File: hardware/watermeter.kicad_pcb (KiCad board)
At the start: 2 copper layers, 100.3 x 49.5 mm, 46 parts, among them J1 flow_meter, J2 t_in, J3 t_out, J4 USB-TYPE-C-31-M-12, J9 24V_Power, SW1 Reboot, U1 K7805-500R3, U2 ESP32-C6-MINI-1, U3 USBLC6-2SC6, U4 LM3671MFX-3.3/NOPB

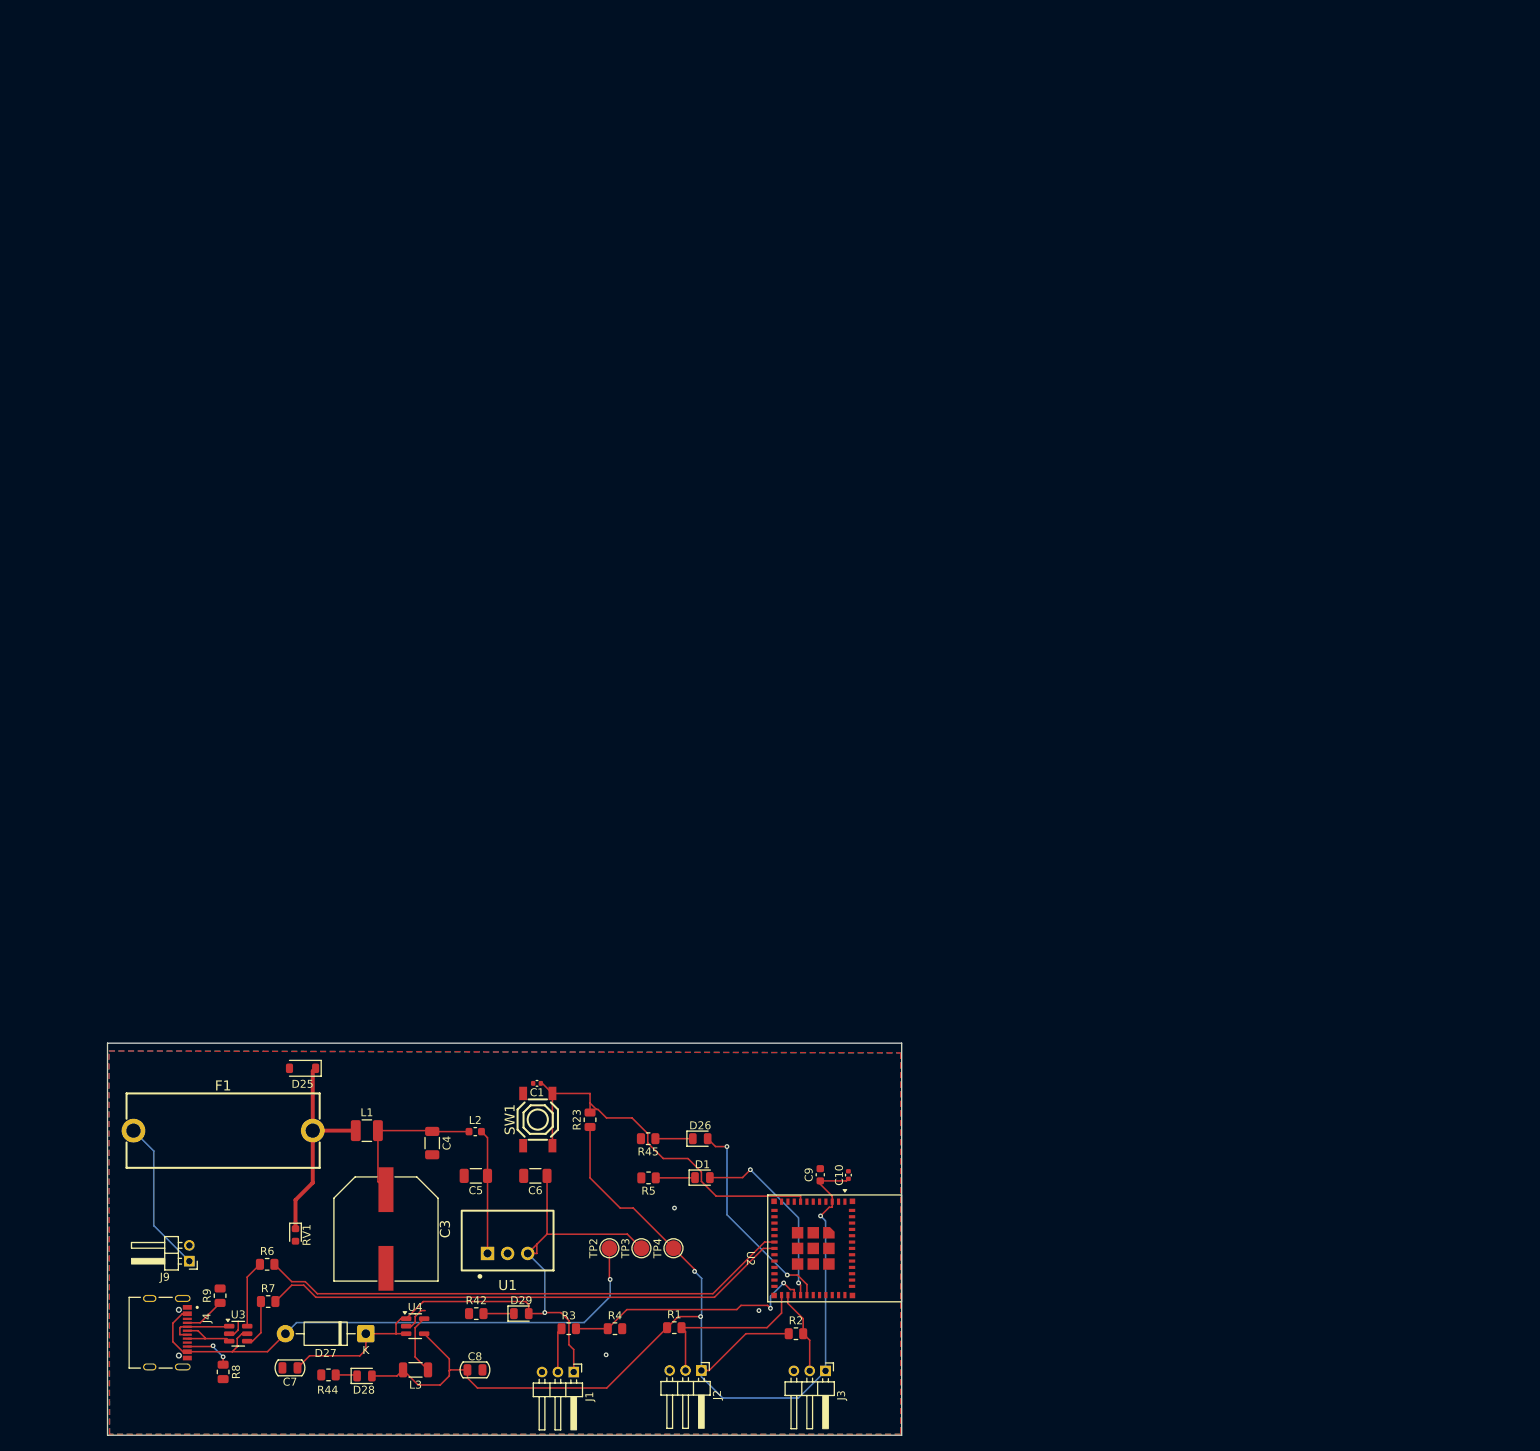
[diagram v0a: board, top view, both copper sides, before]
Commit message: Refactoring
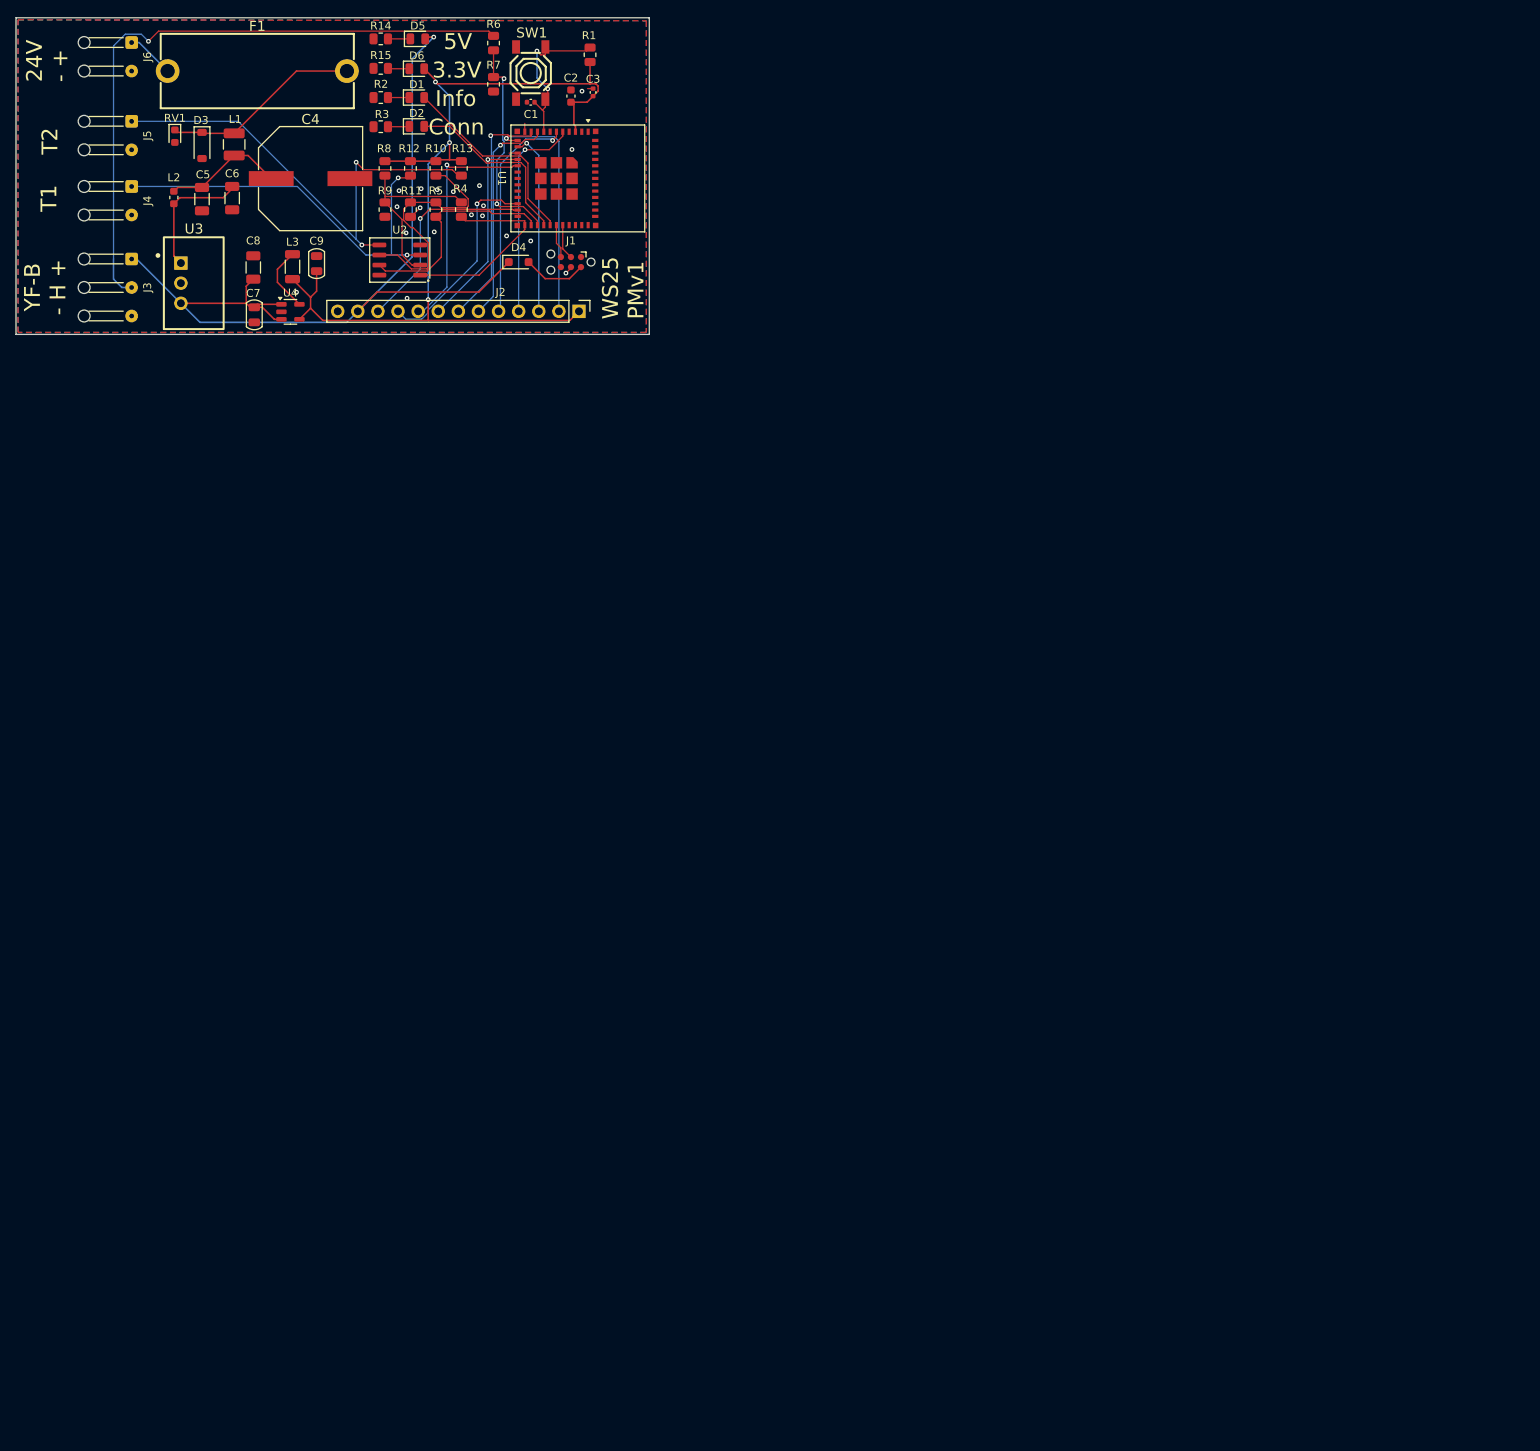
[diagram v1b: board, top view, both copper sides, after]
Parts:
- removed C10: 0.1uF, Capacitor_SMD:C_0402_1005Metric
- removed D25: BAT46W, Diode_SMD:D_SOD-123
- removed D26, D28, D29: KT-0805G, LED_SMD:LED_0805_2012Metric
- removed D27: 1N5819, Diode_THT:D_DO-41_SOD81_P10.16mm_Horizontal
- removed J9: 24V_Power, Connector_PinHeader_2.00mm:PinHeader_1x02_P2.00mm_Horizontal
- removed R23: 10K, Resistor_SMD:R_0805_2012Metric
- removed R42, R44, R45: 20R, Resistor_SMD:R_0805_2012Metric
- removed TP2: 5V_USB, TestPoint:TestPoint_Pad_D2.0mm
- removed TP3: 5V, TestPoint:TestPoint_Pad_D2.0mm
- removed TP4: 3.3V, TestPoint:TestPoint_Pad_D2.0mm
- added C2: 22uF, Capacitor_SMD:C_0603_1608Metric, F.Cu at (70.1, 9.89)
- added D2: KT-0805B, Diode_SMD:D_0805_2012Metric, F.Cu at (50.6, 13.7)
- added D3: BAT46W, Diode_SMD:D_SOD-123, F.Cu at (23.5, 16.1)
- added D4: 1N5819, Diode_SMD:D_SOD-323_HandSoldering, F.Cu at (63.5, 30.9)
- added D5: KT-0805G, LED_SMD:LED_0805_2012Metric, F.Cu at (50.8, 2.67)
- added D6: KT-0805G, LED_SMD:LED_0805_2012Metric, F.Cu at (50.6, 6.44)
- added J5: PT1000-2, Connector_Wire:SolderWire-0.1sqmm_1x02_P3.6mm_D0.4mm_OD1mm_Relief, F.Cu at (14.6, 13.1)
- added J6: 24V_Power, Connector_Wire:SolderWire-0.1sqmm_1x02_P3.6mm_D0.4mm_OD1mm_Relief, F.Cu at (14.6, 3.13)
- added R10: 4k7, Resistor_SMD:R_0805_2012Metric, F.Cu at (53.0, 19.0)
- added R11: 1k, Resistor_SMD:R_0805_2012Metric, F.Cu at (49.8, 24.2)
- added R12: 4k7, Resistor_SMD:R_0805_2012Metric, F.Cu at (49.8, 19.0)
- added R13: 4k7, Resistor_SMD:R_0805_2012Metric, F.Cu at (56.3, 19.0)
- added R14: 20R, Resistor_SMD:R_0805_2012Metric, F.Cu at (46.1, 2.67)
- added R15: 20R, Resistor_SMD:R_0805_2012Metric, F.Cu at (46.1, 6.39)
- C3: value 680uF/50V -> 0.1uF; footprint MyFootprints:CAP-SMD_BD12.5-L13.0-W13.0-LS14.4-FD -> Capacitor_SMD:C_0402_1005Metric
- C4: value 4.7uF/63V -> 680uF/50V; footprint Capacitor_SMD:C_1206_3216Metric -> MyFootprints:CAP-SMD_BD12.5-L13.0-W13.0-LS14.4-FD
- C5: value 10uF/50V -> 4.7uF/63V
- C6: value 22uF/10V -> 10uF/50V
- C8: value 10uF -> 22uF/10V; footprint PCM_Capacitor_SMD_AKL:C_0805_2012Metric -> Capacitor_SMD:C_1206_3216Metric
- C9: value 22uF -> 10uF; footprint Capacitor_SMD:C_0603_1608Metric -> PCM_Capacitor_SMD_AKL:C_0805_2012Metric
- D1: value KT-0805B -> KT-0805G; footprint Diode_SMD:D_0805_2012Metric -> LED_SMD:LED_0805_2012Metric
- J1: value flow_meter -> TC2030; footprint Connector_PinHeader_2.00mm:PinHeader_1x03_P2.00mm_Horizontal -> Connector:Tag-Connect_TC2030-IDC-NL_2x03_P1.27mm_Vertical
- J2: value t_in -> EXT; footprint Connector_PinHeader_2.00mm:PinHeader_1x03_P2.00mm_Horizontal -> Connector_PinHeader_2.54mm:PinHeader_1x13_P2.54mm_Vertical
- J3: value t_out -> flow_meter; footprint Connector_PinHeader_2.00mm:PinHeader_1x03_P2.00mm_Horizontal -> Connector_Wire:SolderWire-0.1sqmm_1x03_P3.6mm_D0.4mm_OD1mm_Relief
- J4: value USB-TYPE-C-31-M-12 -> PT1000-1; footprint MyFootprints:USB-HRO_TYPE-C-31-M-12 -> Connector_Wire:SolderWire-0.1sqmm_1x02_P3.6mm_D0.4mm_OD1mm_Relief
- R1: value 3.3k -> 10K
- R2: value 3.3k -> 20R
- R3: value 1k -> 15R
- R4: value 2k -> 20k
- R5: value 15R -> 20k
- R6: value 22R -> 1k
- R7: value 22R -> 2k
- R8: value 5.1 -> 4k7
- R9: value 5.1 -> 1k
- U1: value K7805-500R3 -> ESP32-C6-MINI-1; footprint MyFootprints:PWRM-TH_K78XX-500R3 -> RF_Module:ESP32-C6-MINI-1
- U2: value ESP32-C6-MINI-1 -> TLV2462AID; footprint RF_Module:ESP32-C6-MINI-1 -> PCM_Package_SO_AKL:SO-8_3.9x4.9mm_P1.27mm
- U3: value USBLC6-2SC6 -> K7805-500R3; footprint Package_TO_SOT_SMD:SOT-23-6 -> MyFootprints:PWRM-TH_K78XX-500R3
- moved J3 165.6 mm to (14.6, 30.5)
- moved R2 164.7 mm to (46.1, 10.1), turned to 180 degrees
- moved R1 161.2 mm to (72.5, 4.68), turned to 90 degrees
- moved R6 156.9 mm to (60.3, 3.20), turned to -90 degrees
- moved R7 156.4 mm to (60.3, 8.41), turned to -90 degrees
- moved R3 153.7 mm to (46.1, 13.8), turned to 180 degrees
- moved R8 153.4 mm to (46.6, 19.0)
- moved C3 146.0 mm to (72.9, 9.43), turned to 90 degrees
- moved J4 144.8 mm to (14.6, 21.3)
- moved R4 142.7 mm to (56.3, 24.2), turned to -90 degrees
- moved C8 142.1 mm to (30.0, 31.5), turned to 90 degrees
- moved D1 141.1 mm to (50.6, 10.1)
- moved L3 140.2 mm to (34.9, 31.4), turned to -90 degrees
- moved J1 140.2 mm to (70.1, 30.9), turned to 180 degrees
- moved RV1 139.6 mm to (20.1, 15.0)
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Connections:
- C1 pad 1: Net-(U2-EN) -> Net-(U1-EN)
- C3 pad 1: Net-(C3-Pad1) -> +3.3V
- C4 pad 1: Net-(C3-Pad1) -> Net-(C4-Pad1)
- C5 pad 1: Net-(U1-IN) -> Net-(C4-Pad1)
- C6 pad 1: +5V -> Net-(U3-IN)
- C8 pad 1: +3.3V -> +5V
- F1 pad 1: Net-(J9-Pin_1) -> /Power/24V
- J1 pad 1: +5V -> /EN
- J1 pad 2: Net-(J1-Pin_2) -> /5V_USB
- J1 pad 3: GND -> /TXD
- J2 pad 3: GND -> Net-(J2-Pin_3)
- J3 pad 1: +3.3V -> +5V
- L1 pad 2: Net-(C3-Pad1) -> Net-(C4-Pad1)
- L2 pad 1: Net-(C3-Pad1) -> Net-(C4-Pad1)
- L2 pad 2: Net-(U1-IN) -> Net-(U3-IN)
- R1 pad 2: Net-(J2-Pin_2) -> Net-(U1-EN)
- R2 pad 1: +3.3V -> Net-(D1-K)
- R2 pad 2: Net-(J3-Pin_2) -> GND
- R3 pad 1: Net-(J1-Pin_2) -> Net-(D2-K)
- R3 pad 2: Net-(U2-IO21) -> GND
- R4 pad 1: Net-(U2-IO21) -> Net-(U2A--)
- R4 pad 2: GND -> Net-(U1-IO19)
- R5 pad 1: Net-(D1-K) -> Net-(U2B--)
- R5 pad 2: GND -> Net-(U1-IO20)
- R6 pad 1: Net-(R6-Pad1) -> Net-(J3-Pin_2)
- R6 pad 2: /USB_D_N -> Net-(U1-IO21)
- R7 pad 1: Net-(R7-Pad1) -> Net-(U1-IO21)
- R7 pad 2: /USB_D_P -> GND
- R8 pad 1: Net-(J4-CC2) -> +3.3V
- R8 pad 2: GND -> Net-(U2A--)
- R9 pad 1: Net-(J4-CC1) -> Net-(U2A--)
- SW1 pad 2: Net-(U2-EN) -> Net-(U1-EN)
- U1 pad 1: Net-(U1-IN) -> GND
- U1 pad 3: +5V -> +3.3V
- U2 pad 1: GND -> Net-(U1-IO19)
- U2 pad 2: GND -> Net-(U2A--)
- U2 pad 3: +3.3V -> Net-(J4-Pin_1)
- U2 pad 5: unconnected-(U2-IO2-Pad5) -> Net-(J5-Pin_1)
- U2 pad 6: unconnected-(U2-IO3-Pad6) -> Net-(U2B--)
- U2 pad 7: unconnected-(U2-NC-Pad7) -> Net-(U1-IO20)
- U2 pad 8: Net-(U2-EN) -> unconnected-(U2A-V+-Pad8)
- U3 pad 1: /D- -> Net-(U3-IN)
- U3 pad 3: /D+ -> +5V
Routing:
- net Net-(J3-Pin_2): track 10.7 -> 82.0 mm, vias 0 -> 1
- net /USB_D_N: track 67.4 -> 0.00 mm
- net /USB_D_P: track 67.1 -> 0.00 mm
- net /5V_USB: track 72.9 -> 8.10 mm, vias 1 -> 0
- net Net-(J5-Pin_1): track 0.00 -> 61.5 mm, vias 0 -> 2
- net Net-(J4-Pin_1): track 0.00 -> 51.8 mm, vias 0 -> 2
- net Net-(U2-EN): track 49.3 -> 0.00 mm
- net Net-(U2-IO21): track 32.2 -> 0.00 mm, vias 2 -> 0
- net Net-(U2B--): track 0.00 -> 30.9 mm
- net +5V: track 83.7 -> 114.5 mm
- net +3.3V: track 154.1 -> 123.4 mm
- net Net-(J2-Pin_7): track 0.00 -> 29.7 mm, vias 0 -> 1
- net Net-(J2-Pin_9): track 0.00 -> 29.5 mm, vias 0 -> 1
- net Net-(J2-Pin_5): track 0.00 -> 28.0 mm, vias 0 -> 1
- net Net-(J2-Pin_6): track 0.00 -> 27.8 mm, vias 0 -> 1
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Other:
- board size 100.3 x 49.5 mm -> 80 x 40 mm
- board text added: "24V - +"
- board text added: "3.3V"
- board text added: "5V"
- board text added: "Conn"
- board text added: "Info"
- board text added: "T1"
- board text added: "T2"
- board text added: "WS25 PMv1"
- board text added: "YF-B - H +"
